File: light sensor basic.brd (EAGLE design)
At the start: 83.2 x 57.8 mm, 1 part

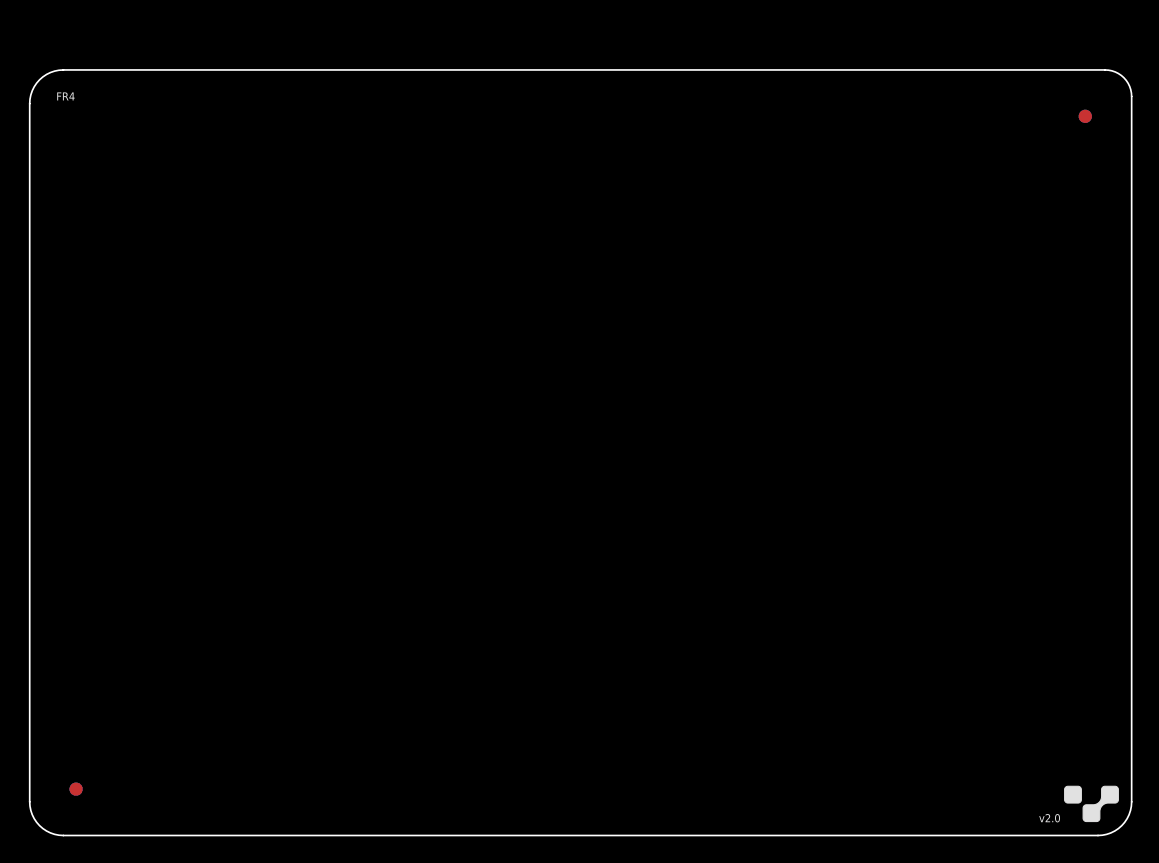
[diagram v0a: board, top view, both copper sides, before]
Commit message: Update board
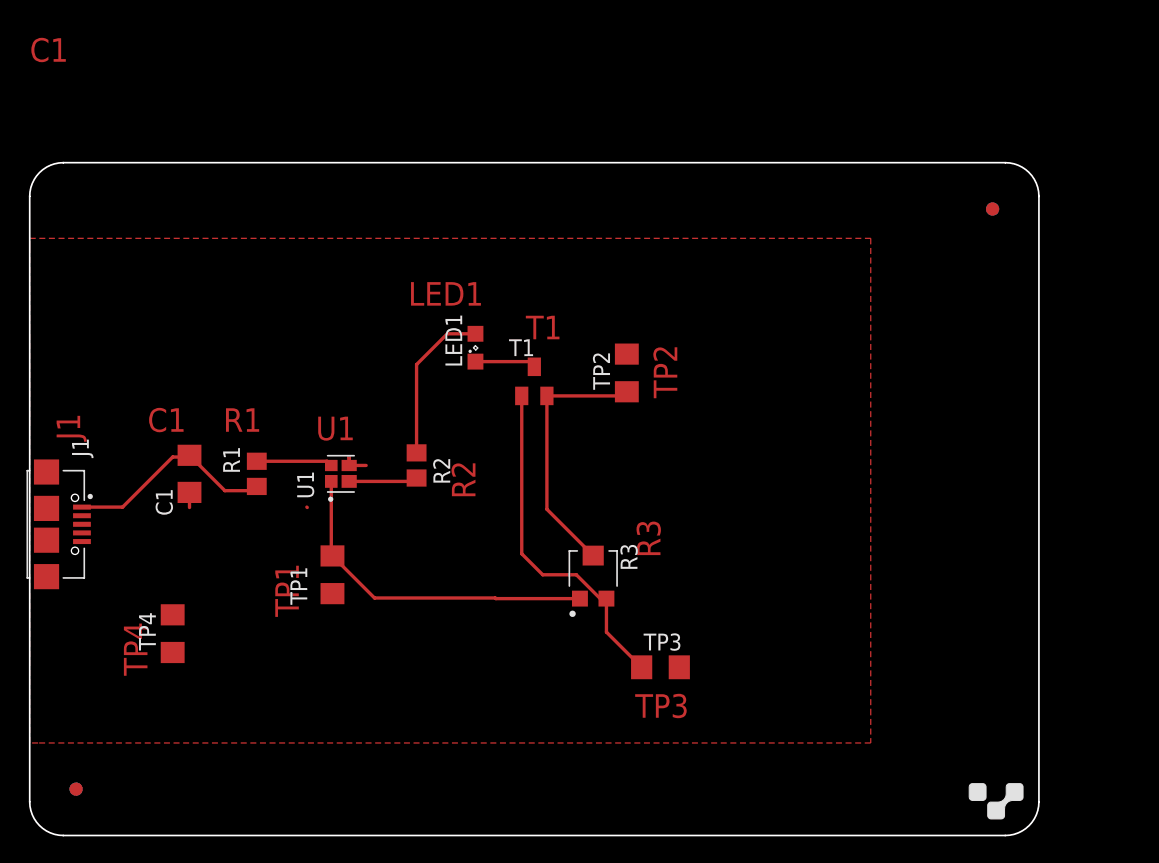
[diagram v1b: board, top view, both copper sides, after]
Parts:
- added C1: 0.1 uF, rcl:C1206
- added J1: UJ2-MIBH-G-SMT-TR, UJ2-MIBH-G-SMT-TR:CUI_UJ2-MIBH-G-SMT-TR
- added LED1: (no value), led:SML0805
- added R1: 82, rcl:R0805
- added R2: 150, rcl:R0805
- added R3: TC33X-2-203E, TC33X-2-203E:TRIM_TC33X-2-203E
- added T1: (no value), transistor:SOT23-EBC
- added TP1, TP2, TP3, TP4: (no value), rcl:R1206
- added U1: VCNT2020, VCNT2020:XDCR_VCNT2020
- U$1: value 2X3_BOARD_V2 -> 2X3_BOARD; device voltera_community_lib:2X3_BOARD_V2 -> voltera_community_lib:2X3_BOARD_V1
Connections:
- new net GND: C1.1, J1.5, J1.S1, J1.S2, J1.S3, J1.S4, R3.3, T1.E, TP3.1, U1.4
- new net N$1: R1.2, U1.3
- new net N$3: R3.1, TP1.1, U1.1
- new net N$4: R3.2, T1.B, TP2.1
- new net N$5: LED1.C, T1.C
- new net N$6: LED1.A, R2.1
- new net VCC: C1.2, J1.1, R1.1, R2.2, TP4.1, U1.2
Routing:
- net GND: track 0.00 -> 30.2 mm
- net N$3: track 0.00 -> 25.7 mm
- net VCC: track 0.00 -> 22.1 mm
- net N$4: track 0.00 -> 19.7 mm
- net N$6: track 0.00 -> 12.1 mm
- net N$1: track 0.00 -> 5.76 mm
- net N$5: track 0.00 -> 4.61 mm
- added copper zone on layer 1, net N$2
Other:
- board size 83.2 x 57.8 mm -> 76.2 x 50.8 mm
- board text added: "C1"
- board text added: "J1"
- board text added: "LED1"
- board text added: "R1"
- board text added: "R2"
- board text added: "R3"
- board text added: "T1"
- board text added: "TP1"
- board text added: "TP2"
- board text added: "TP3"
- board text added: "TP4"
- board text added: "U1"
